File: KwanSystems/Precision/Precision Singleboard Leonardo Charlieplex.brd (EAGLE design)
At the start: 76.2 x 76.2 mm, 273 parts, among them J501 GP-2106, Q501 SSM6N58NU, Q502 SSM6N58NU, U401 ATMEGA32U4TQFP, U501 5319 1.8V, Y401 16MHz

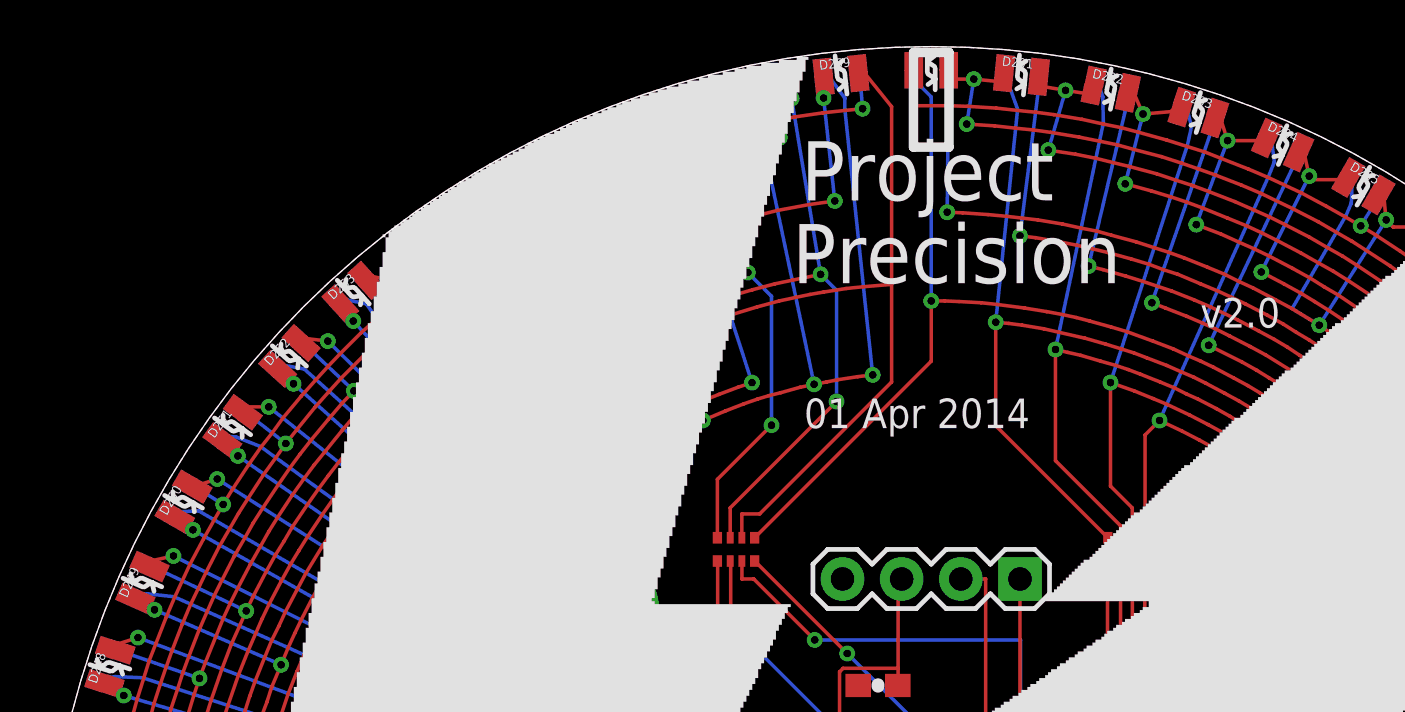
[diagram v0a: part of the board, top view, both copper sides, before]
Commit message: Shuffled several documents
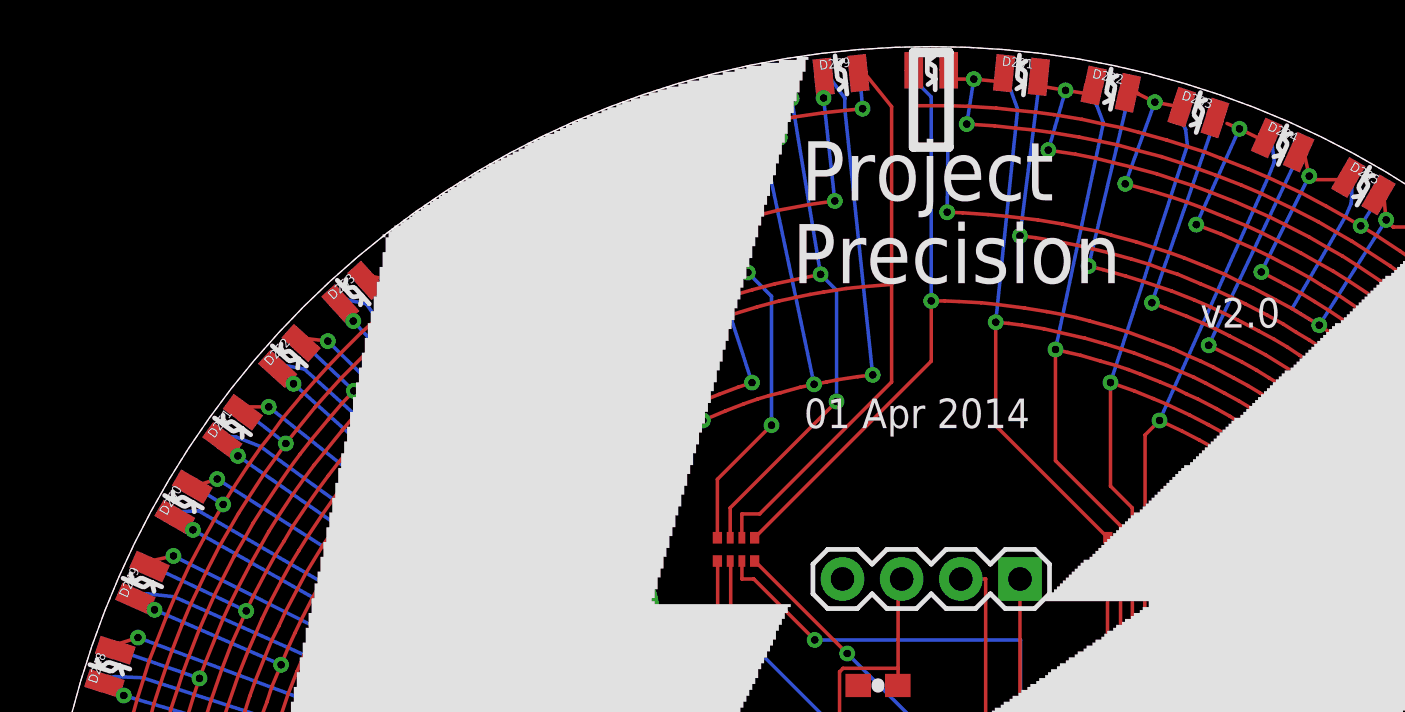
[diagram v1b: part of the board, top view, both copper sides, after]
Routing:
- net Q04: track 269.6 -> 271.0 mm
- net Q10: track 309.8 -> 310.6 mm
- net Q12: track 304.9 -> 305.6 mm
